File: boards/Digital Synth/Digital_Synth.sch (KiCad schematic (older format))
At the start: 33 parts, among them J5 Barrel_Jack, J6 JTAG, J7 Micro_SD_Card, SW1 SW_Push, SW2 SW_Push, U1 LM1117-3.3, U5 STM32F405RGTx, U7 Adafruit_2in, Y1 8MHz

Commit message: almost done with layout
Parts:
- removed C2, C9: 1uF, symbol device:C_Small
- removed J7: Micro_SD_Card, symbol Connector:Micro_SD_Card
- removed SW2: SW_Push, Button_Switch_THT:SW_PUSH_6mm, symbol Switch:SW_Push
- removed U7: Adafruit_2in, Display:Adafruit_2in, symbol Display_Graphic:Adafruit_2in
- added C2, C9: 10uF, Capacitor_THT:CP_Radial_D5.0mm_P2.00mm, symbol device:CP_Small
- added J7: UART_Debug, Connector_PinHeader_2.54mm:PinHeader_1x02_P2.54mm_Vertical, symbol Connector:Conn_01x02_Male
- added J9: UART_MIDI, Connector_PinHeader_2.54mm:PinHeader_1x02_P2.54mm_Vertical, symbol Connector:Conn_01x02_Male
- added U8: Adafruit_2.4in, Display:Adafruit_2.4in, symbol Display_Graphic:Adafruit_2.4in
- D31, D32, D33: footprint (none) -> Diode_SMD:D_0805_2012Metric_Pad1.15x1.40mm_HandSolder
- J5: value Barrel_Jack -> 5V IN; footprint (none) -> Connector_BarrelJack:BarrelJack_CUI_PJ-102AH_Horizontal
- R10, R11, R9: value R_Small -> 470; footprint (none) -> Resistor_SMD:R_0603_1608Metric_Pad1.05x0.95mm_HandSolder
- R12, R8: footprint Resistor_SMD:R_0805_2012Metric_Pad1.15x1.40mm_HandSolder -> Resistor_SMD:R_0603_1608Metric_Pad1.05x0.95mm_HandSolder
- R13: footprint (none) -> Resistor_SMD:R_0603_1608Metric_Pad1.05x0.95mm_HandSolder
- TP1: footprint (none) -> TestPoint:TestPoint_Pad_1.0x1.0mm
- U1: footprint (none) -> Package_TO_SOT_SMD:SOT-223
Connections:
- net +3V3: now also C9.1
- net +5V: now also C2.1, U8.2 (Vin)
- net BCK: now also U5.51 (PC10); no longer U5.34 (PB13)
- net GND: now also C2.2, C9.2, U8.1 (GND)
- net MCK: now also U5.38 (PC7); no longer U5.37 (PC6)
- net SD: now also U5.53 (PC12); no longer U5.36 (PB15)
- net SPI2_CS: now also U5.33 (PB12)
- net SPI2_MISO: now also U5.35 (PB14)
- net SPI2_MOSI: now also U5.36 (PB15)
- net SPI2_SCK: now also U5.34 (PB13)
- net WS: now also U5.50 (PA15); no longer U5.33 (PB12)
- net B8: now reaches U5.10 (PC2)
- net B9: now reaches U5.11 (PC3)
- net RV1: now reaches U5.14 (PA0)
- net RV2: now reaches U5.15 (PA1)
- net RV3: now reaches U5.16 (PA2)
- net RV4: now reaches U5.17 (PA3)
- net B3: now reaches U5.2 (PC13)
- net RV5: now reaches U5.20 (PA4)
- net RV6: now reaches U5.21 (PA5)
- net RV7: now reaches U5.22 (PA6)
- net RV8: now reaches U5.23 (PA7)
- net Y+: now reaches U5.24 (PC4)
- net Y+: now also U8.11 (Y+)
- net X+: now reaches U5.25 (PC5)
- net X+: now also U8.12 (X+)
- net Y-: now reaches U5.26 (PB0)
- net Y-: now also U8.13 (Y-)
- net X-: now reaches U5.27 (PB1)
- net X-: now also U8.14 (X-)
- net TX_Debug: now reaches U5.29 (PB10)
- net TX_Debug: now also J7.1 (Pin_1)
- net B4: now reaches U5.3 (PC14)
- net RX_Debug: now reaches U5.30 (PB11)
- net RX_Debug: now also J7.2 (Pin_2)
- net B5: now reaches U5.4 (PC15)
- net TX_MIDI: now reaches U5.42 (PA9)
- net TX_MIDI: now also J9.1 (Pin_1)
- net RX_MIDI: now reaches U5.43 (PA10)
- net RX_MIDI: now also J9.2 (Pin_2)
- net at U5.44 (PA11): now also R9.1
- net at U5.45 (PA12): now also R10.1
- net SPI1_SCK: now reaches U5.55 (PB3)
- net SPI1_SCK: now also U8.4 (CLK)
- net SPI1_MISO: now reaches U5.56 (PB4)
- net SPI1_MISO: now also U8.5 (MISO)
- net SPI1_MOSI: now reaches U5.57 (PB5)
- net SPI1_MOSI: now also U8.6 (MOSI)
- net SPI1_CS2: now reaches U5.58 (PB6)
- net SPI1_CS2: now also U8.7 (CS)
- net SPI1_CS1: now reaches U5.59 (PB7)
- net SPI1_CS1: now also U8.19 (CCS)
- net at R12.1, U5.60 (BOOT0): now also TP1.1
- net B1: now reaches U5.61 (PB8)
- net B2: now reaches U5.62 (PB9)
- net B6: now reaches U5.8 (PC0)
- net B7: now reaches U5.9 (PC1)
- net SDIO_CMD renamed DC
- net DC: now also U8.8 (D/C)
- no-connect marks 1 -> 30
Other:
- note added: "Analog"
- note added: "I2S_CK"
- note removed: "I2S_CLK"
- moved on the sheet: C10, C11, C12, C13, C15, C17, C21, C25, C26, C27, C3, C6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

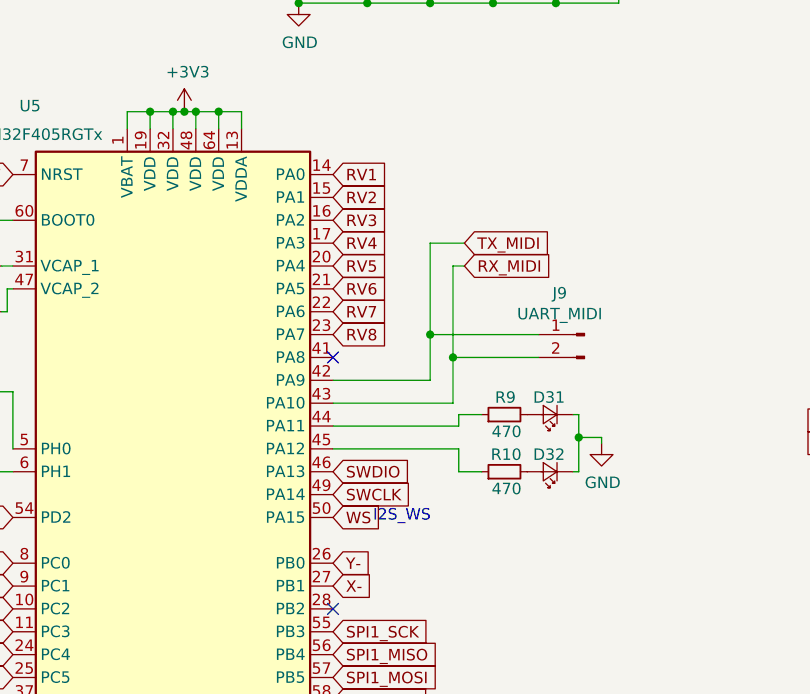
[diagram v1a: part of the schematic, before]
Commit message: finished layout
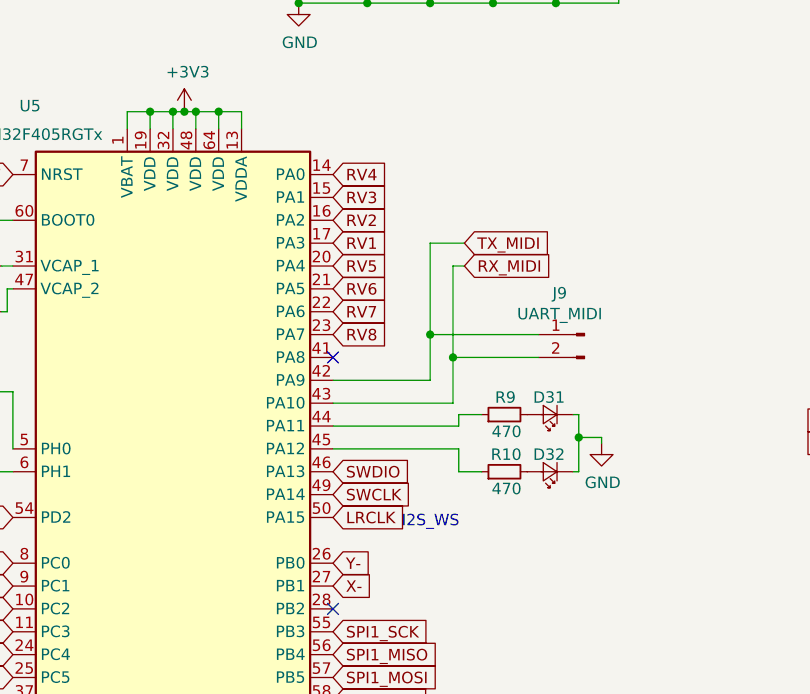
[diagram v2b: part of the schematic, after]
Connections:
- net RV1: now also U5.17 (PA3); no longer U5.14 (PA0)
- net RV2: now also U5.16 (PA2); no longer U5.15 (PA1)
- net RV3: now also U5.15 (PA1); no longer U5.16 (PA2)
- net RV4: now also U5.14 (PA0); no longer U5.17 (PA3)
- net WS renamed LRCLK
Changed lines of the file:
@@
 Text Notes 4875 5175 2    50   ~ 0
 I2S_CK
-Text Notes 6700 3975 0    50   ~ 0
+Text Notes 6825 4000 0    50   ~ 0
 I2S_WS
 Text Notes 4525 4875 0    50   ~ 0
@@
 Text GLabel 5125 5150 0    50   Input ~ 0
 BCK
-Text GLabel 6525 3950 2    50   Input ~ 0
-WS
 $Comp
 L power:+5V #PWR07
@@
 Text GLabel 5125 4450 0    50   Input ~ 0
 B9
+Text GLabel 6525 2750 2    50   Input ~ 0
+RV1
+Text GLabel 6525 2650 2    50   Input ~ 0
+RV2
+Text GLabel 6525 2550 2    50   Input ~ 0
+RV3
 Text GLabel 6525 2450 2    50   Input ~ 0
-RV1
-Text GLabel 6525 2550 2    50   Input ~ 0
-RV2
-Text GLabel 6525 2650 2    50   Input ~ 0
-RV3
-Text GLabel 6525 2750 2    50   Input ~ 0
 RV4
 Text GLabel 6525 2850 2    50   Input ~ 0
@@
 Wire Wire Line
 	4725 2650 5125 2650
+Text GLabel 6525 3950 2    50   Input ~ 0
+LRCLK
 $EndSCHEMATC
